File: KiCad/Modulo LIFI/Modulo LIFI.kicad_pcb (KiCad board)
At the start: 2 copper layers, 23 x 14 mm, 8 parts, among them J2 Arduino NANO, U3 LM358

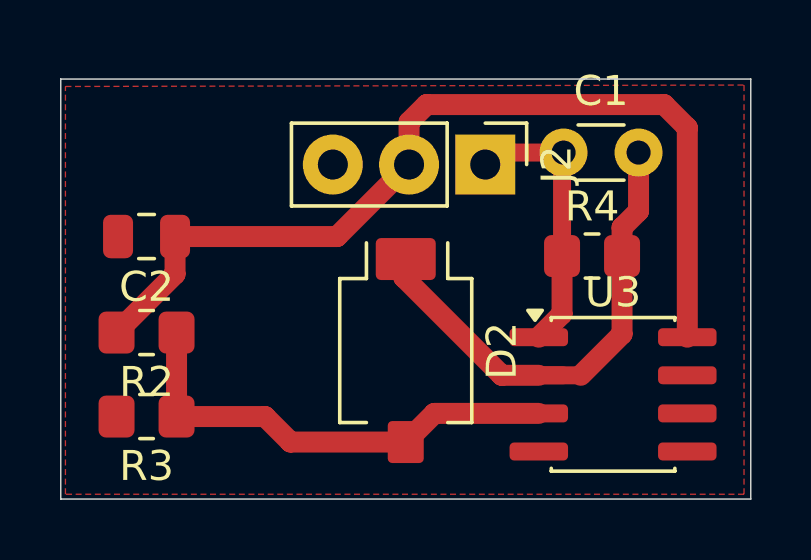
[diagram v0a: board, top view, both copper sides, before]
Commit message: Mensaje describiendo tus cambios
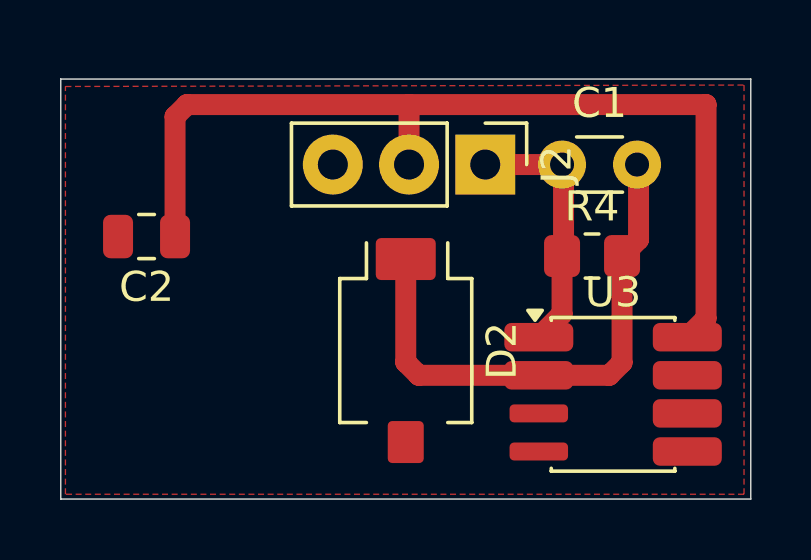
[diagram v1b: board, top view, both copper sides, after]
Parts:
- removed R2, R3: 100k, Resistor_SMD:R_0805_2012Metric_Pad1.20x1.40mm_HandSolder
- C1: value 100nf -> 22pf
- R4: value 22k -> 1Mhoms
- moved C1 0.40 mm to (18.3, 4.60)
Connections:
- D2 pad 2: Net-(D2-A) -> GND
- U3 pad 3: Net-(D2-A) -> GND
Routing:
- net Net-(D2-A): track 15.6 -> 0.00 mm
- net Net-(D2-K): track 16.3 -> 18.2 mm
- net +5V: track 31.0 -> 31.9 mm
